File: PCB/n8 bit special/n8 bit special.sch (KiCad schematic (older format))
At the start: 36 parts, among them J1 USB_B_Micro, J2 PORT0, J3 PORT2, J4 PORT1, J5 PORT3, J6 Conn_02x08_Odd_Even, SW1 SW_Push_Dual, U1 W65C02SxP, U2 CY62256-70PC, U3 CY62256-70PC, U4 28C256, U5 74LS21, U6 22V10C, U7 DS1813, X1 4Mhz

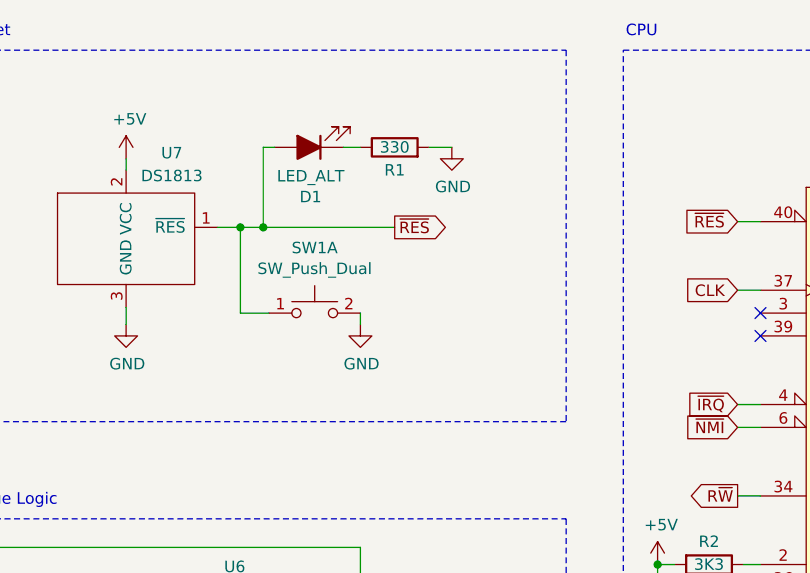
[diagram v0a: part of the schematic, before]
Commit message: More v2 changes
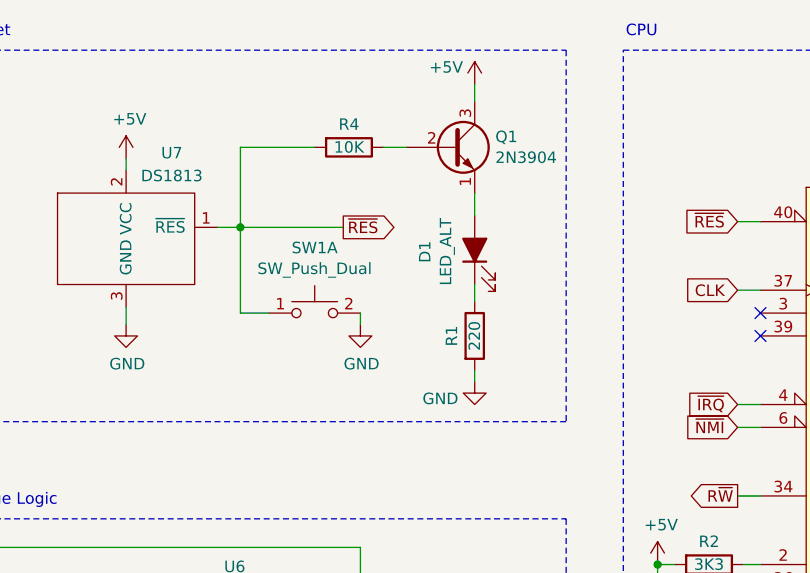
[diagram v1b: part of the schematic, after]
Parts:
- added Q1: 2N3904, Package_TO_SOT_THT:TO-92, symbol Transistor_BJT:2N3904
- added R4: 10K, Resistor_THT:R_Axial_DIN0207_L6.3mm_D2.5mm_P7.62mm_Horizontal, symbol Device:R
- R1: value 330 -> 220
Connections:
- net +5V: now also Q1.3 (C)
- net ~RES: now also R4.2; no longer D1.2 (A)
- new net: D1.2 (A), Q1.1 (E)
- new net: Q1.2 (B), R4.1
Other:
- moved on the sheet: D1, R1
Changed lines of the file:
@@
 	1    0    0    -1
 $EndComp
-Text GLabel 4650 1650 2    50   Output ~ 0
+Text GLabel 4425 1650 2    50   Output ~ 0
 ~RES
 $Comp
@@
 L Device:LED_ALT D1
 U 1 1 6045033F
-P 4275 1300
-F 0 "D1" H 4268 1517 50  0000 C CNN
-F 1 "LED_ALT" H 4268 1426 50  0000 C CNN
-F 2 "LED_THT:LED_D3.0mm" H 4275 1300 50  0001 C CNN
-F 3 "~" H 4275 1300 50  0001 C CNN
-	1    4275 1300
-	-1   0    0    1
+P 5000 1750
+F 0 "D1" H 4993 1967 50  0000 C CNN
+F 1 "LED_ALT" H 4993 1876 50  0000 C CNN
+F 2 "LED_THT:LED_D3.0mm" H 5000 1750 50  0001 C CNN
+F 3 "~" H 5000 1750 50  0001 C CNN
+	1    5000 1750
+	0    -1   -1   0
 $EndComp
 $Comp
 L power:GND #PWR0128
 U 1 1 60450336
-P 4900 1300
-F 0 "#PWR0128" H 4900 1050 50  0001 C CNN
-F 1 "GND" H 4905 1127 50  0000 C CNN
-F 2 "" H 4900 1300 50  0001 C CNN
-F 3 "" H 4900 1300 50  0001 C CNN
-	1    4900 1300
+P 5000 2325
+F 0 "#PWR0128" H 5000 2075 50  0001 C CNN
+F 1 "GND" H 4850 2250 50  0000 C CNN
+F 2 "" H 5000 2325 50  0001 C CNN
+F 3 "" H 5000 2325 50  0001 C CNN
+	1    5000 2325
 	1    0    0    -1
 $EndComp
@@
 L Device:R R1
 U 1 1 60450330
-P 4650 1300
-F 0 "R1" V 4550 1300 50  0000 C CNN
-F 1 "330" V 4650 1300 50  0000 C CNN
-F 2 "Resistor_THT:R_Axial_DIN0207_L6.3mm_D2.5mm_P7.62mm_Horizontal" H 4650 1300 50  0001 C CNN
-F 3 "~" H 4650 1300 50  0001 C CNN
-	1    4650 1300
-	0    -1   -1   0
-$EndComp
-Wire Wire Line
-	4425 1300 4500 1300
-Wire Wire Line
-	4800 1300 4900 1300
+P 5000 2125
+F 0 "R1" V 4900 2125 50  0000 C CNN
+F 1 "220" V 5000 2125 50  0000 C CNN
+F 2 "Resistor_THT:R_Axial_DIN0207_L6.3mm_D2.5mm_P7.62mm_Horizontal" H 5000 2125 50  0001 C CNN
+F 3 "~" H 5000 2125 50  0001 C CNN
+	1    5000 2125
+	1    0    0    -1
+$EndComp
+Wire Wire Line
+	5000 1900 5000 1975
+Wire Wire Line
+	5000 2275 5000 2325
 Wire Notes Line
 	8550 875  8550 3900
@@
 Connection ~ 3975 1650
 Wire Wire Line
-	3975 1650 4075 1650
-Wire Wire Line
 	4500 2025 4500 2075
-Wire Wire Line
-	4075 1300 4075 1650
-Connection ~ 4075 1650
-Wire Wire Line
-	4075 1650 4650 1650
-Wire Wire Line
-	4075 1300 4125 1300
 Wire Notes Line
 	5400 875  5400 2500
@@
 	1625 4275 1625 4300
 NoConn ~ 950  2075
+Wire Wire Line
+	3975 1650 4425 1650
+$Comp
+L Transistor_BJT:2N3904 Q1
+U 1 1 60DCF972
+P 4900 1300
+F 0 "Q1" H 5090 1346 50  0000 L CNN
+F 1 "2N3904" H 5090 1255 50  0000 L CNN
+F 2 "Package_TO_SOT_THT:TO-92" H 5100 1225 50  0001 L CIN
+F 3 "https://www.onsemi.com/pub/Collateral/2N3903-D.PDF" H 4900 1300 50  0001 L CNN
+	1    4900 1300
+	1    0    0    -1
+$EndComp
+Wire Wire Line
+	4600 1300 4700 1300
+$Comp
+L power:+5V #PWR01
+U 1 1 611B59A4
+P 5000 1025
+F 0 "#PWR01" H 5000 875 50  0001 C CNN
+F 1 "+5V" H 4875 1100 50  0000 C CNN
+F 2 "" H 5000 1025 50  0001 C CNN
+F 3 "" H 5000 1025 50  0001 C CNN
+	1    5000 1025
+	1    0    0    -1
+$EndComp
+Wire Wire Line
+	5000 1025 5000 1100
+Wire Wire Line
+	5000 1500 5000 1600
+$Comp
+L Device:R R4
+U 1 1 60DD1216
+P 4450 1300
+F 0 "R4" V 4350 1300 50  0000 C CNN
+F 1 "10K" V 4450 1300 50  0000 C CNN
+F 2 "Resistor_THT:R_Axial_DIN0207_L6.3mm_D2.5mm_P7.62mm_Horizontal" H 4450 1300 50  0001 C CNN
+F 3 "~" H 4450 1300 50  0001 C CNN
+	1    4450 1300
+	0    1    1    0
+$EndComp
+Wire Wire Line
+	3975 1650 3975 1300
+Wire Wire Line
+	3975 1300 4300 1300
 Wire Bus Line
 	6375 8950 6375 9450
